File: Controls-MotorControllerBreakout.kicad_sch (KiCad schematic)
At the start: 13 parts, among them J1 MC CAN 1, J2 MC CAN 2, J3 CTRLS, J4 EXT PWR, J5 CANDAPTER

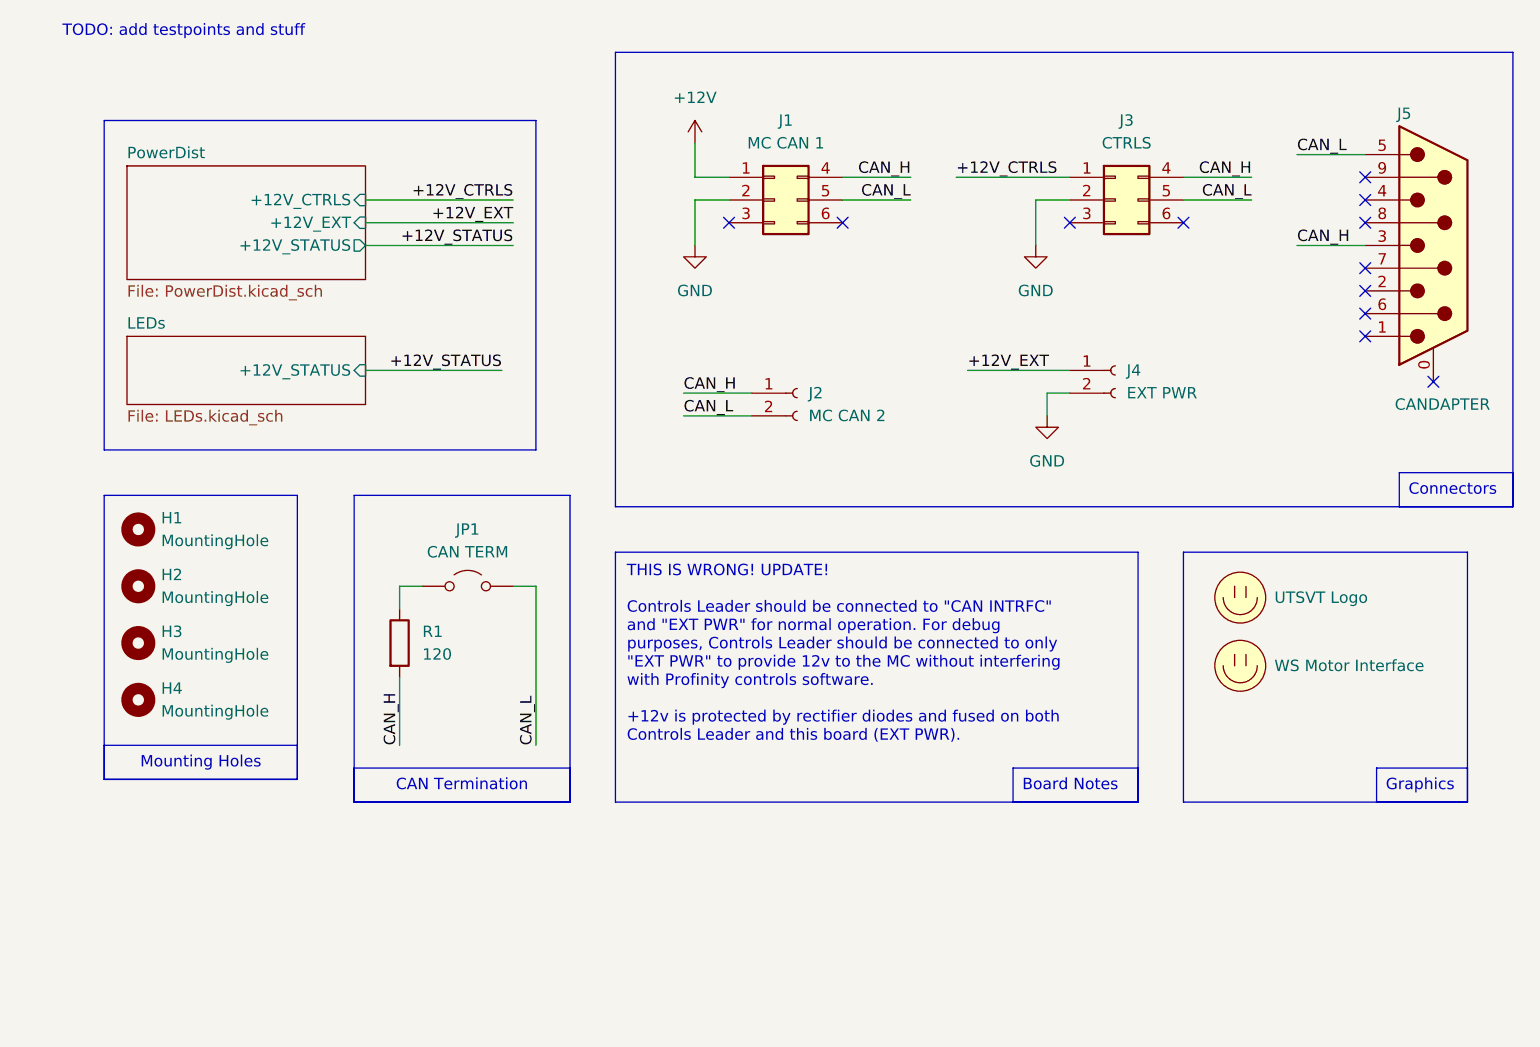
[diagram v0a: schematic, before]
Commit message: yap
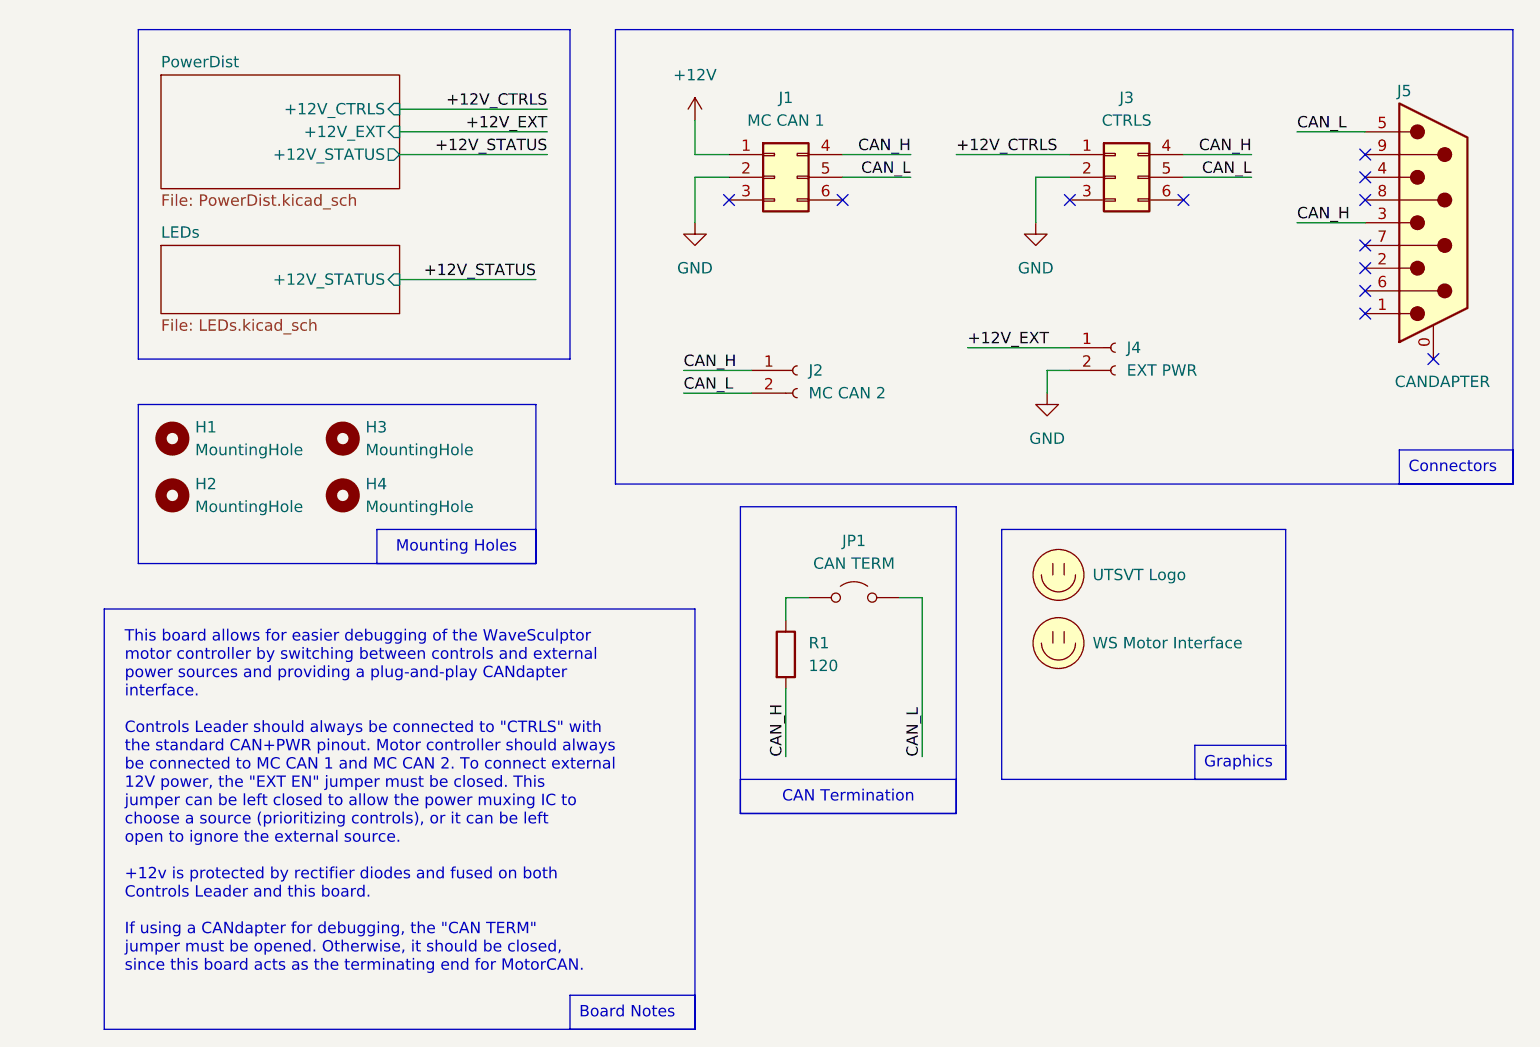
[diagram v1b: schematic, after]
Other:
- note added: "This board allows for easier debugging of the WaveSculptor motor controller by switching between controls and external power sources and providing a plug-and-play CANdapter interface. Controls Leader should always be connected to "CTRLS" with the standard CAN+PWR pinout. Motor controller should always be connected to MC CAN 1 and MC CAN 2. To connect external 12V power, the "EXT EN" jumper must b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"
- note removed: "THIS IS WRONG! UPDATE! Controls Leader should be connected to "CAN INTRFC" and "EXT PWR" for normal operation. For debug purposes, Controls Leader should be connected to only "EXT PWR" to provide 12v to the MC without interfering with Profinity controls software. +12v is protected by rectifier diodes and fused on both Controls Leader and this board (EXT PWR)."
- note removed: "TODO: add testpoints and stuff"
- moved on the sheet: H1, H2, H3, H4, J1, J2, J3, J4, J5, JP1, R1
